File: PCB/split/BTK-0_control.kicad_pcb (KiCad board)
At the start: 4 copper layers, 22 x 51.5 mm, 27 parts, among them J1 USB_C_Receptacle_USB2.0_16P, J6 Conn_01x16_Pin, SW1 EN, SW2 BOOT, U1 NCP1117-3.3_SOT223, U2 NCP1117-3.3_SOT223, U3 USBLC6-2SC6, U4 ESP32-C6-MINI-1, U5 TVS1400DRV

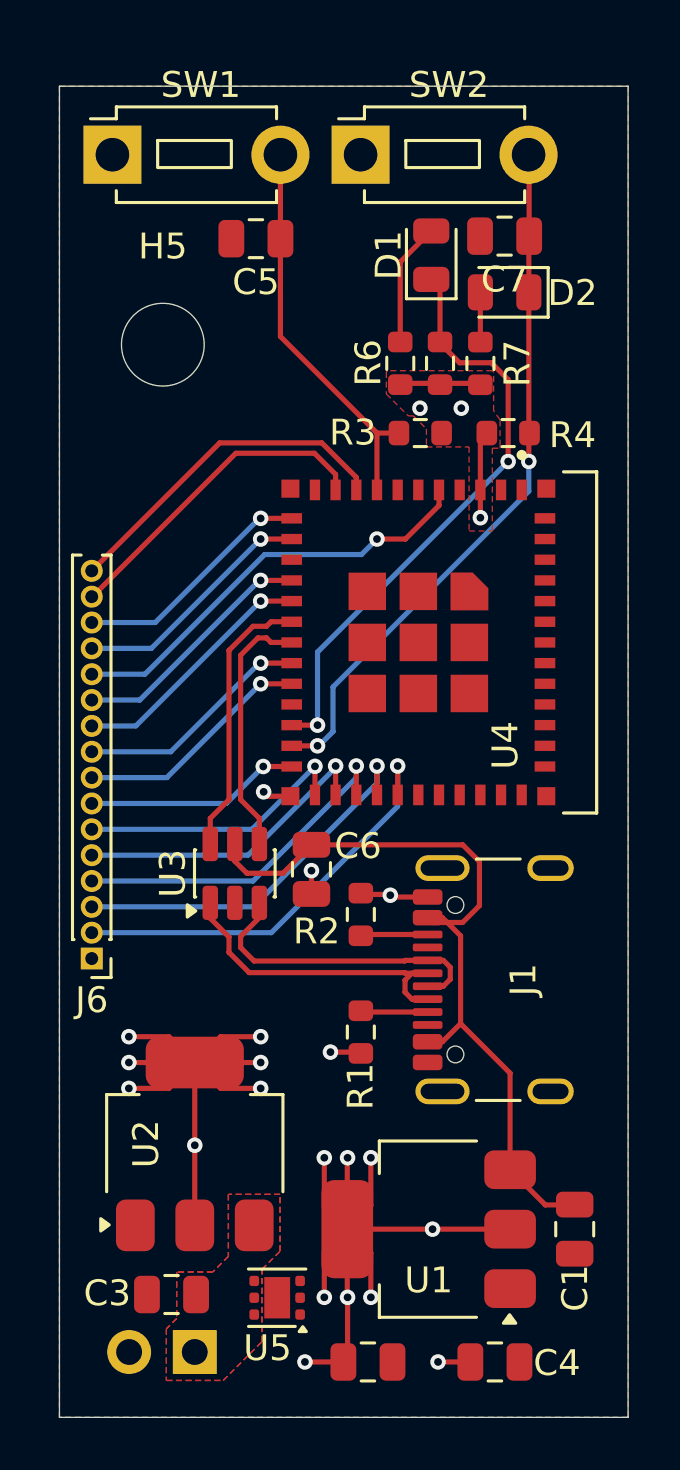
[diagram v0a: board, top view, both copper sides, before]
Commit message: im boutta die son
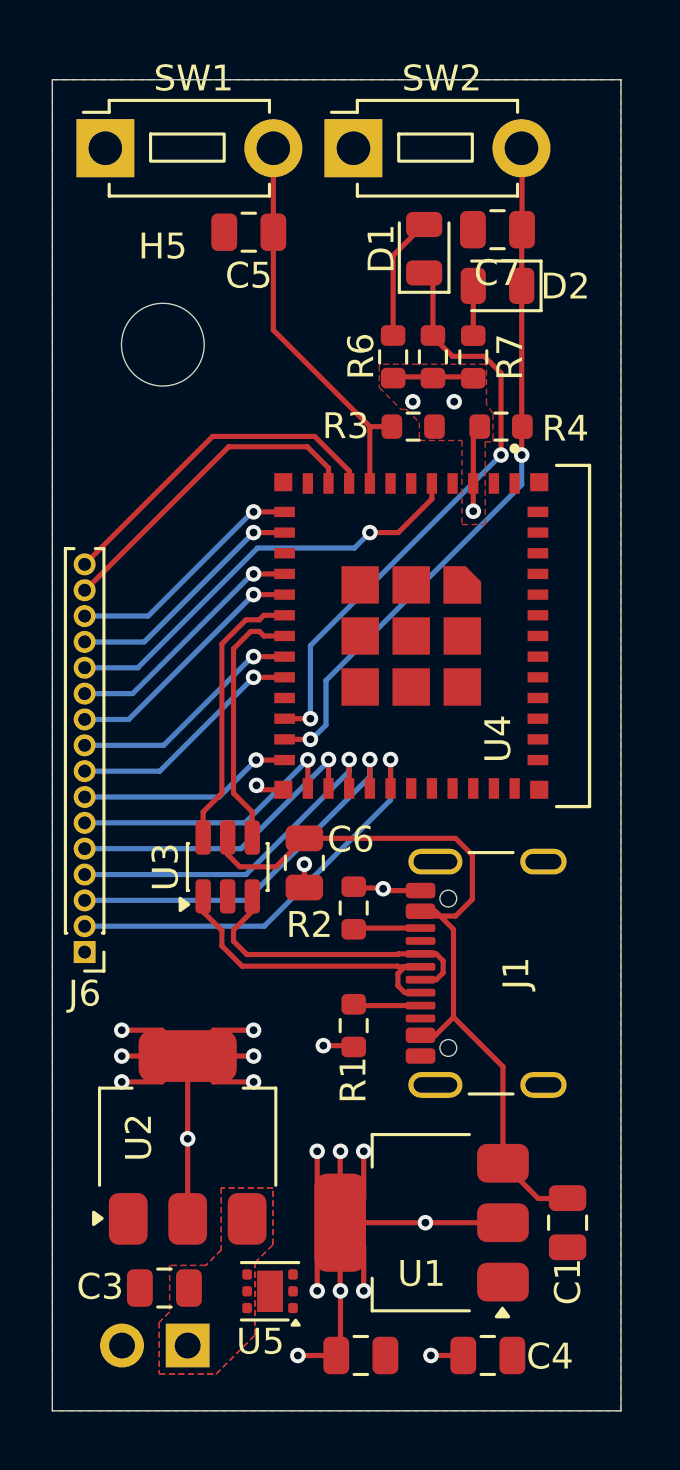
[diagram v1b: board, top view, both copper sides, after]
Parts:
- moved C1 0.37 mm to (15.7, 34.0)
- moved C4 0.37 mm to (12.6, 39.1)
- moved C6 0.37 mm to (5.47, 20.1)
- moved C7 0.37 mm to (12.9, -4.45)
- moved D1 0.37 mm to (10.1, -3.71)
- moved D2 0.37 mm to (12.9, -2.27)
- moved J1 0.37 mm to (13.7, 24.3)
- moved R1 0.37 mm to (7.38, 26.3)
- moved R2 0.37 mm to (7.38, 21.8)
- moved R3 0.37 mm to (9.69, 3.17)
- moved R5 0.37 mm to (10.4, 0.47)
- moved R6 0.37 mm to (8.91, 0.47)
- moved R7 0.37 mm to (12.0, 0.48)
- moved SW2 0.37 mm to (7.38, -7.60)
- moved U1 0.37 mm to (10.0, 34.0)
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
